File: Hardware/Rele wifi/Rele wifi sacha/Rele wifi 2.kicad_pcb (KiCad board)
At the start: 2 copper layers, 65 x 50 mm, 16 parts, among them J1 Screw_Terminal_01x02, J2 Screw_Terminal_01x03, J4 Conn_01x03_Pin, K1 G5LE-1, Q2 BC337, SW1 SW_Push, U5 PC817

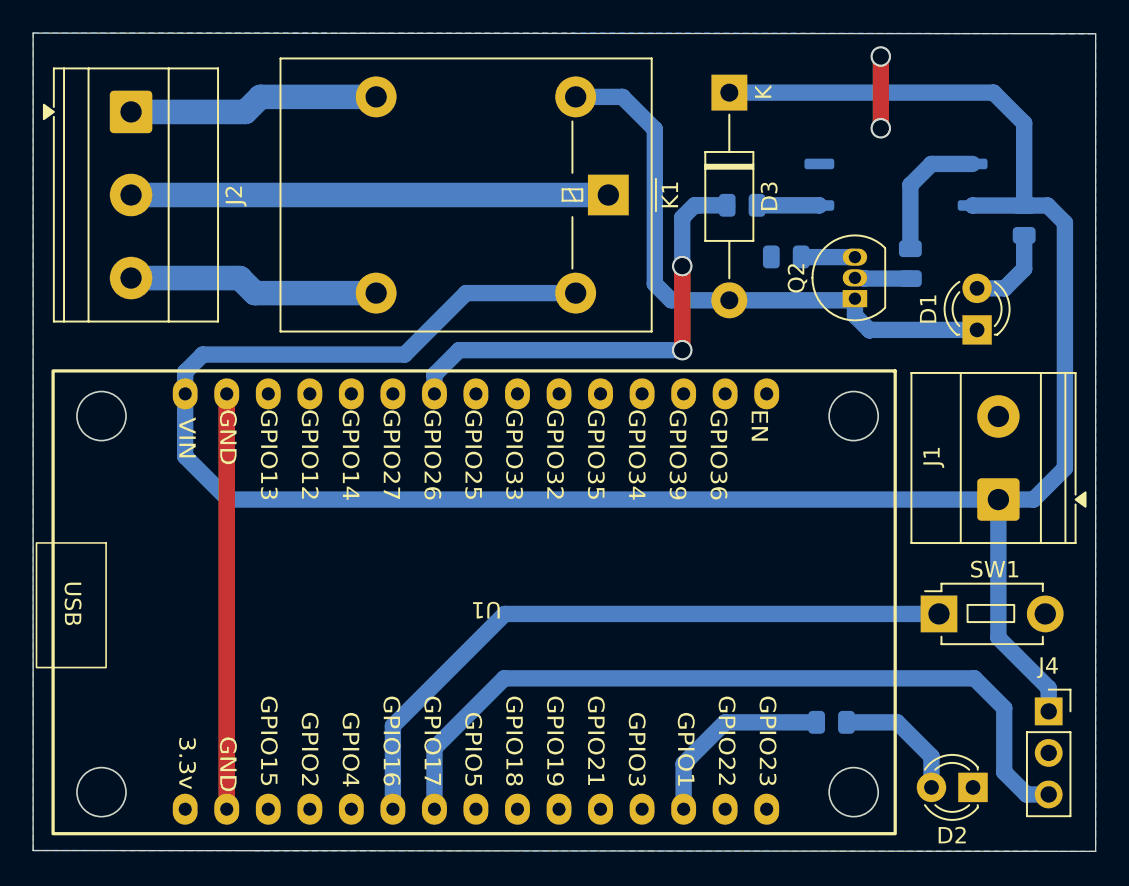
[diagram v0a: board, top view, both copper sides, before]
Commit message: actu pcb
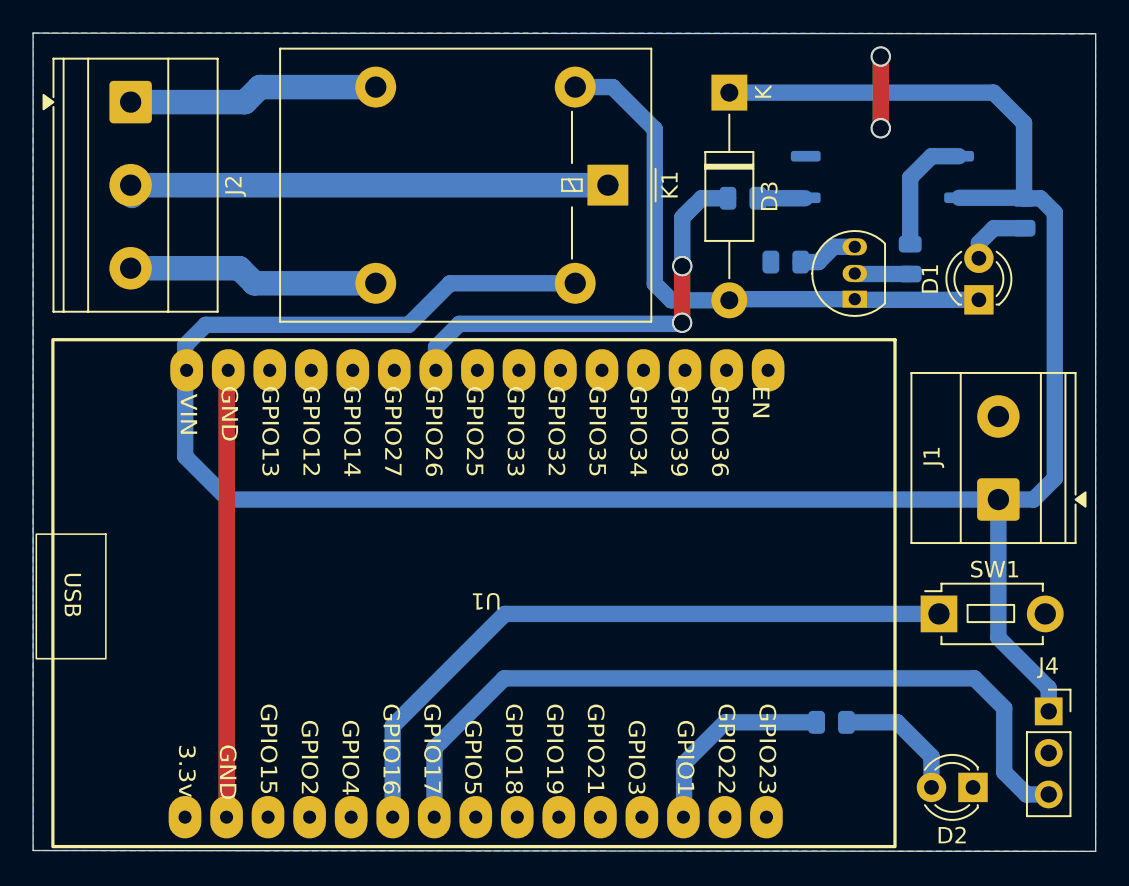
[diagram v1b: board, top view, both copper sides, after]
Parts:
- moved D1 1.84 mm to (210.2, 53.3)
- moved U5 0.95 mm to (204.3, 45.8)
- moved J2 0.60 mm to (158.3, 41.2)
- moved K1 0.60 mm to (187.5, 46.3)
- moved U1 0.54 mm to (178.6, 70.4)
- moved R1 0.44 mm to (212.9, 48.0)
- moved R3 0.43 mm to (195.8, 47.1)
- moved R4 0.31 mm to (198.4, 51.0)
- moved R2 0.28 mm to (206.0, 50.8)
- moved Q2 0.27 mm to (202.6, 52.9)
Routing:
- net GND: track 29.8 -> 31.8 mm
- net +5V: track 146.0 -> 147.5 mm
- net Net-(D1-A): track 5.42 -> 4.07 mm
- net Net-(R3-Pad2): track 3.81 -> 2.90 mm
- net Net-(R2-Pad1): track 8.24 -> 7.60 mm
- net Net-(Q2-B): track 2.89 -> 3.40 mm
